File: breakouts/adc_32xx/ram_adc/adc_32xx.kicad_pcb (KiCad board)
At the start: 4 copper layers, 78 x 38.5 mm, 102 parts, among them J201 Conn_Coaxial, J202 Conn_Coaxial, J203 Conn_02x06_Odd_Even, J204 Conn_02x20_Odd_Even, J205 Conn_01x07, J301 Conn_Coaxial, J401 Conn_Coaxial, J501 Conn_01x01, J502 Conn_01x01, T301 MABAES0060, T302 MABAES0060, T401 MABAES0060, T402 MABAES0060, U201 VEMI65AB-HCI, U202 ADC322x, U501 ADM7170

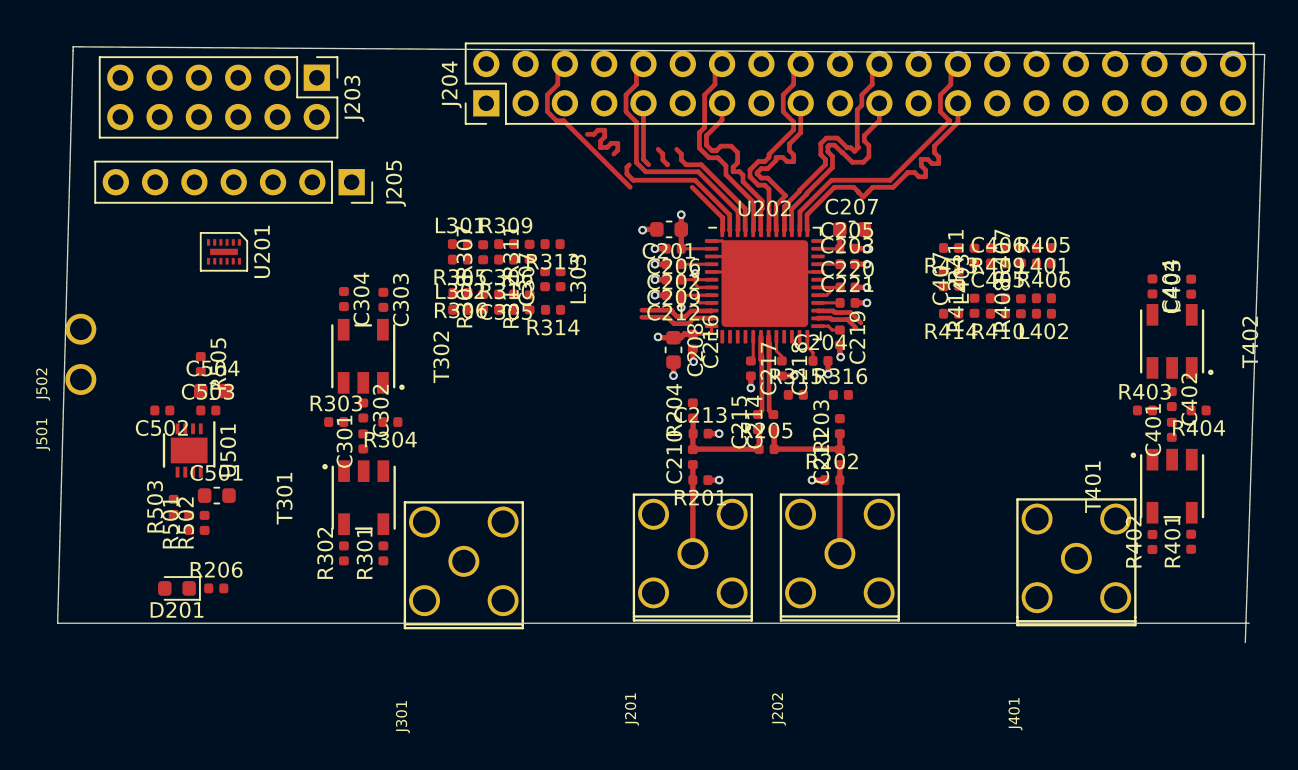
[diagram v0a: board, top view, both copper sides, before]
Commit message: finished layout of adc32xx ecp5 board
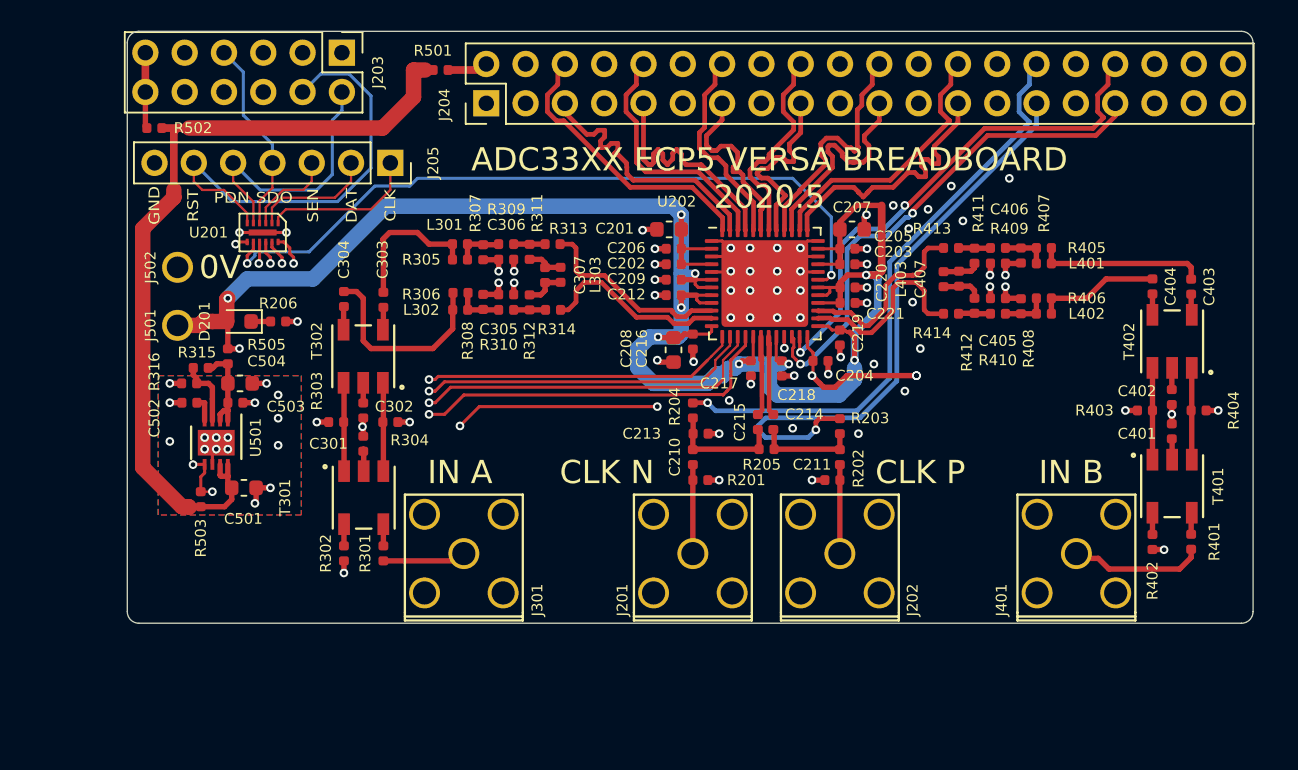
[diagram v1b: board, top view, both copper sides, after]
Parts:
- added G***: LOGO, vna_footprints:cat, B.Cu at (97.8, 57.5)
- moved R316 42.1 mm to (49.0, 61.5), turned to 180 degrees
- moved R315 38.5 mm to (49.8, 60.5), turned to 180 degrees
- moved R501 33.5 mm to (65.2, 41.2), turned to 180 degrees
- moved R502 25.7 mm to (46.8, 45.0), turned to 0 degrees
- moved D201 17.7 mm to (52.2, 57.5)
- moved R206 17.7 mm to (54.8, 57.5)
- moved J502 7.42 mm to (48.2, 54.0)
- moved J501 7.16 mm to (48.2, 57.8)
- moved J205 2.80 mm to (62.0, 47.2)
- moved U201 2.80 mm to (53.8, 51.8)
- moved J203 2.29 mm to (58.9, 40.1)
- moved C501 1.82 mm to (52.5, 68.2)
- moved C502 1.82 mm to (49.0, 62.8)
- moved C503 1.82 mm to (52.0, 62.8)
- moved C504 1.82 mm to (52.3, 61.5)
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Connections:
- U501 pad 6: (no net) -> GND
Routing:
- net +1V8: track 31.5 -> 128.8 mm, vias 4 -> 10
- net Net-(C501-Pad1): track 0.00 -> 53.7 mm
- net /VCM: track 1.71 -> 54.9 mm, vias 0 -> 7
- net Net-(U201-Pad7): track 0.00 -> 48.2 mm, vias 0 -> 4
- net Net-(U201-Pad8): track 0.00 -> 47.5 mm, vias 0 -> 2
- net Net-(U201-Pad9): track 0.00 -> 42.4 mm, vias 0 -> 2
- net Net-(U201-Pad10): track 0.00 -> 40.3 mm, vias 0 -> 2
- net /adc/CLK_FPGA_N: track 0.00 -> 38.6 mm, vias 0 -> 1
- net /adc/CLK_FPGA_P: track 0.00 -> 38.5 mm, vias 0 -> 1
- net Net-(U201-Pad11): track 0.00 -> 38.0 mm, vias 0 -> 2
- net Net-(U201-Pad12): track 0.00 -> 36.1 mm, vias 0 -> 2
- net /adc/SYSREF_N: track 0.04 -> 33.7 mm, vias 0 -> 2
- net /adc/SYSREF_P: track 0.04 -> 32.8 mm, vias 0 -> 2
- net /adc/EN: track 0.00 -> 31.9 mm, vias 0 -> 2
- net /adc/RESET: track 0.00 -> 29.7 mm
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- added copper zone on B.Cu, net GND
- added copper zone on F.Cu, net GND
- added copper zone on In2.Cu, net GND
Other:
- board size 78 x 38.5 mm -> 72.8 x 38.2 mm
- rule solder_mask_min_width: 0.25 -> 0.15
- board text added: "0V"
- board text added: "ADC33XX ECP5 VERSA BREADBOARD 2020.5"
- board text added: "CLK"
- board text added: "CLK N"
- board text added: "CLK P"
- board text added: "DAT"
- board text added: "GND"
- board text added: "IN A"
- board text added: "IN B"
- board text added: "PDN"
- board text added: "RST"
- board text added: "SDO"
- board text added: "SEN"
